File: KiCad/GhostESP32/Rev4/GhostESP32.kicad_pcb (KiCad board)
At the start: 2 copper layers, 50 parts, among them J1 USB_OTG, J2 CONN_01X12, J3 CONN_01X12, J4 STEERING, J5 MOTOR, Q1 Q_NPN_BEC, Q2 Q_NPN_BEC, Q3 Q_NPN_BEC, Q4 BSS138, Q5 BSS138, SW1 SW_SPDT, U1 NCP1117-3.3_SOT223, U2 CP2102, U3 TMP102, U4 MPU-9250, U5 ESP-WROOM-32

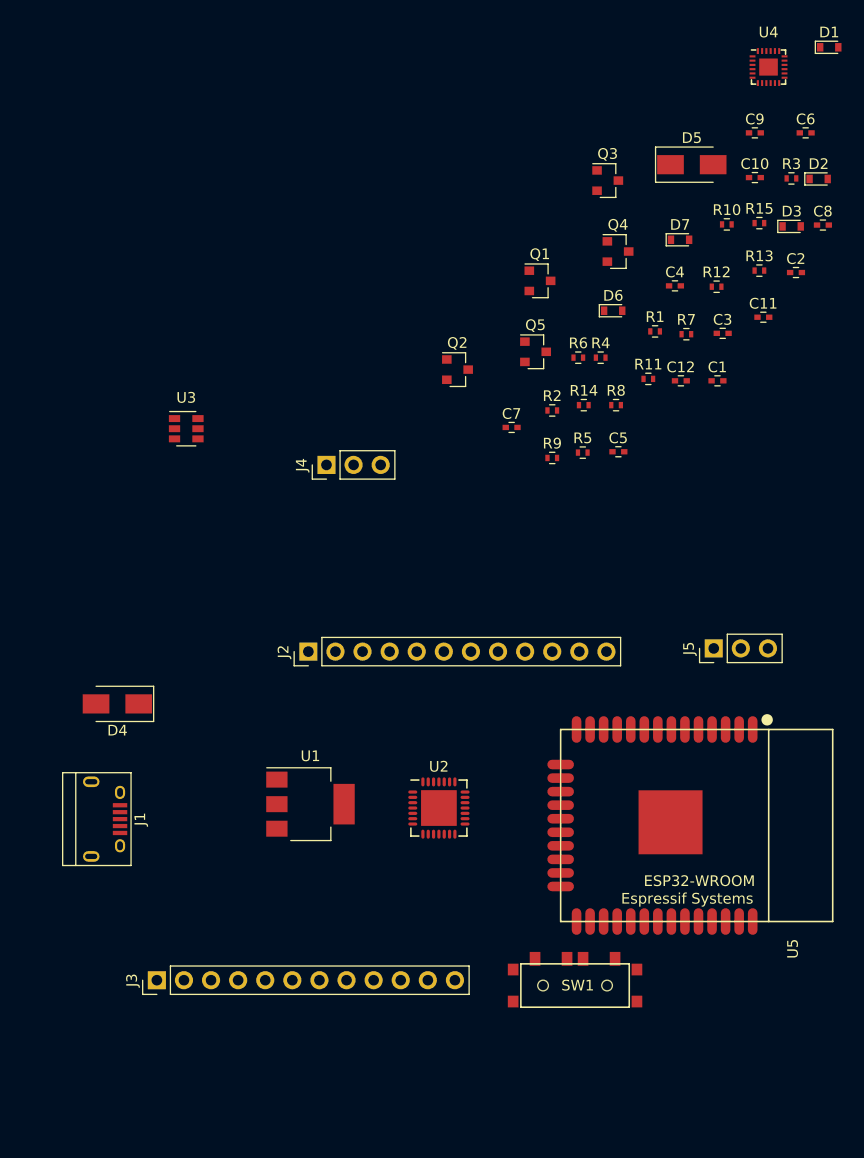
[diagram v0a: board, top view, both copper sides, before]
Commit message: A massive bunch of former changes waiting to be committed.
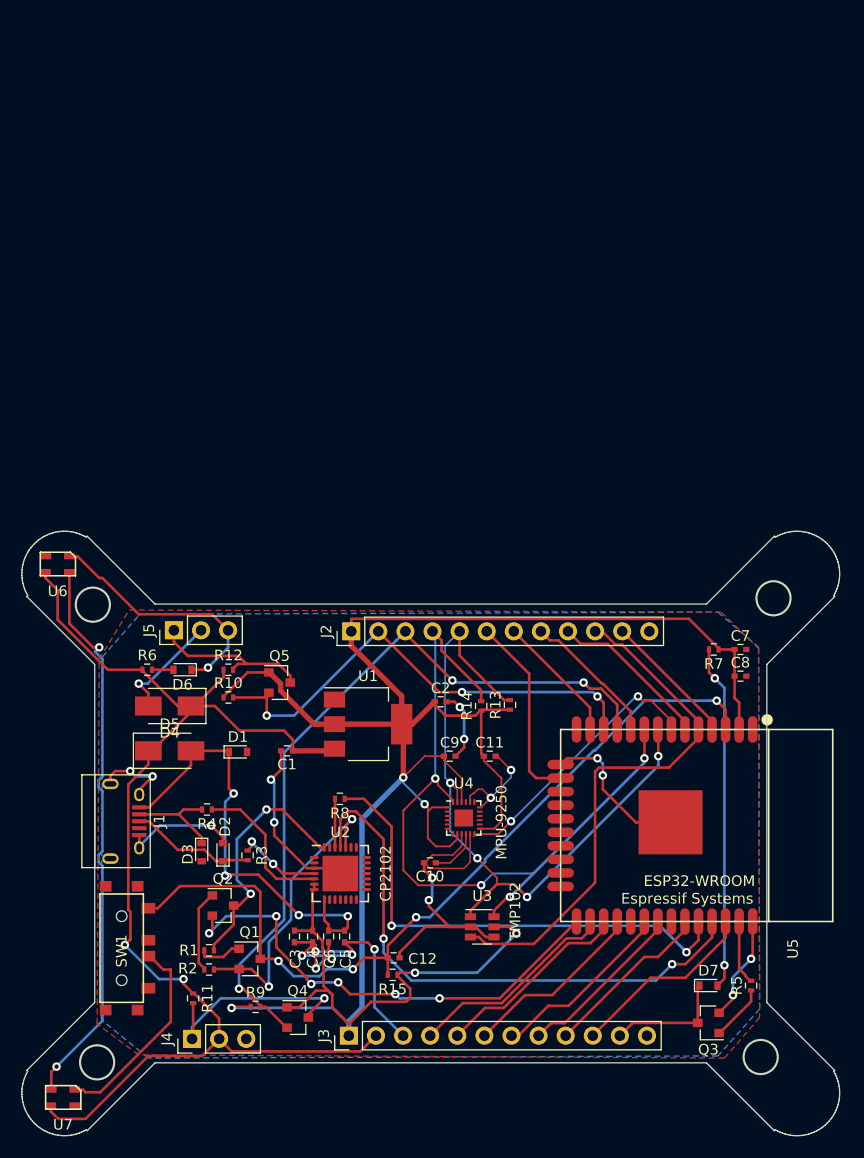
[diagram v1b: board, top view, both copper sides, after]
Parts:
- added U6: NeoPixelNano, NorBotKiCadFootprints:NeoPixelNano, F.Cu at (113.0, 80.5)
- added U7: NeoPixelNano, NorBotKiCadFootprints:NeoPixelNano, F.Cu at (113.5, 130.5)
- moved C6 87.6 mm to (138.4, 115.4), turned to 270 degrees
- moved D1 86.2 mm to (129.9, 98.1)
- moved D2 84.3 mm to (128.5, 107.5), turned to 90 degrees
- moved R3 81.4 mm to (130.8, 107.8), turned to 270 degrees
- moved D3 80.6 mm to (126.5, 107.5), turned to 270 degrees
- moved Q3 79.5 mm to (174.0, 123.5), turned to 180 degrees
- moved R15 78.4 mm to (144.4, 119.0), turned to 180 degrees
- moved Q4 77.8 mm to (135.5, 123.0)
- moved U4 76.0 mm to (151.1, 104.3)
- moved D5 73.6 mm to (123.5, 98.0)
- moved R11 72.1 mm to (125.7, 121.2), turned to 270 degrees
- moved R1 71.5 mm to (127.2, 116.7)
- moved C10 71.1 mm to (147.9, 108.5), turned to 180 degrees
- moved D7 70.0 mm to (174.0, 120.0)
- moved C4 69.8 mm to (136.9, 115.4), turned to 270 degrees
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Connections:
- J2 pad 4: IO25 -> IO33/SDA
- J2 pad 5: IO33/SDA -> IO32/SCL
- J2 pad 6: IO32/SCL -> IO13
- J2 pad 8: IO13 -> IO25
- J3 pad 10: IO21 -> IO22
- J3 pad 11: IO22 -> LED
- J3 pad 4: LED -> IO4
- J3 pad 5: IO4 -> IO16
- J3 pad 6: IO16 -> IO17
- J3 pad 7: IO17 -> IO18
- J3 pad 8: IO18 -> IO19
- J3 pad 9: IO19 -> IO21
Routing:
- net +3V3: track 0.00 -> 217.1 mm, vias 0 -> 5
- net GND: track 0.00 -> 182.4 mm, vias 0 -> 22
- net +5V: track 0.00 -> 116.7 mm, vias 0 -> 2
- net EN: track 0.00 -> 77.5 mm, vias 0 -> 4
- net IO33/SDA: track 0.00 -> 71.8 mm, vias 0 -> 4
- net IO26: track 0.00 -> 71.2 mm, vias 0 -> 3
- net IO32/SCL: track 0.00 -> 65.3 mm, vias 0 -> 4
- net RXD: track 0.00 -> 53.7 mm, vias 0 -> 2
- net Net-(U6-Pad1): track 0.00 -> 53.0 mm, vias 0 -> 2
- net I39: track 0.00 -> 50.5 mm
- net TXD: track 0.00 -> 46.8 mm, vias 0 -> 2
- net IO27: track 0.00 -> 45.9 mm, vias 0 -> 3
- net IO0: track 0.00 -> 45.0 mm, vias 0 -> 6
- net VBUS: track 0.00 -> 42.8 mm, vias 0 -> 4
- net Net-(D7-Pad2): track 0.00 -> 32.4 mm, vias 0 -> 2
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- added copper zone on B.Cu, net GND
- added copper zone on F.Cu, net GND
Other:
- board outline added: 76.7 x 56.7 mm
- net class Default: clearance 0 -> 0.2
- rule trace_clearance: 0 -> 0.2
- rule trace_min: 0.2 -> 0.15
- board text added: "+5V"
- board text added: "+5V ESC"
- board text added: "3V3"
- board text added: "5V"
- board text added: "CP2102"
- board text added: "GND"
- board text added: "Ghost32 Rev 4 Frode Lillerud 23.aug 2017"
- board text added: "I34"
- board text added: "I36"
- board text added: "I39"
- board text added: "IO13"
- board text added: "IO14"
- board text added: "IO16"
- board text added: "IO17"
- board text added: "IO18"
- board text added: "IO19"
- board text added: "IO21"
- board text added: "IO22"
- board text added: "IO25"
- board text added: "IO26"
- board text added: "IO27"
- board text added: "IO4"
- board text added: "LED"
- board text added: "MOTOR PWM"
- board text added: "MPU-9250"
- board text added: "SCL/IO32"
- board text added: "SDA/IO33"
- board text added: "STEERING PWM"
- board text added: "TMP102"
